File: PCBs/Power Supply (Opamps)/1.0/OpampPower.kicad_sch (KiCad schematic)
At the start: 30 parts, among them J1 Conn_01x02_Male, J2 Conn_01x02_Male, J3 Conn_01x03_Male, J4 Conn_01x03_Male, J5 Conn_01x03_Male, U1 LM317_SOT-223, U2 LM337_SOT223

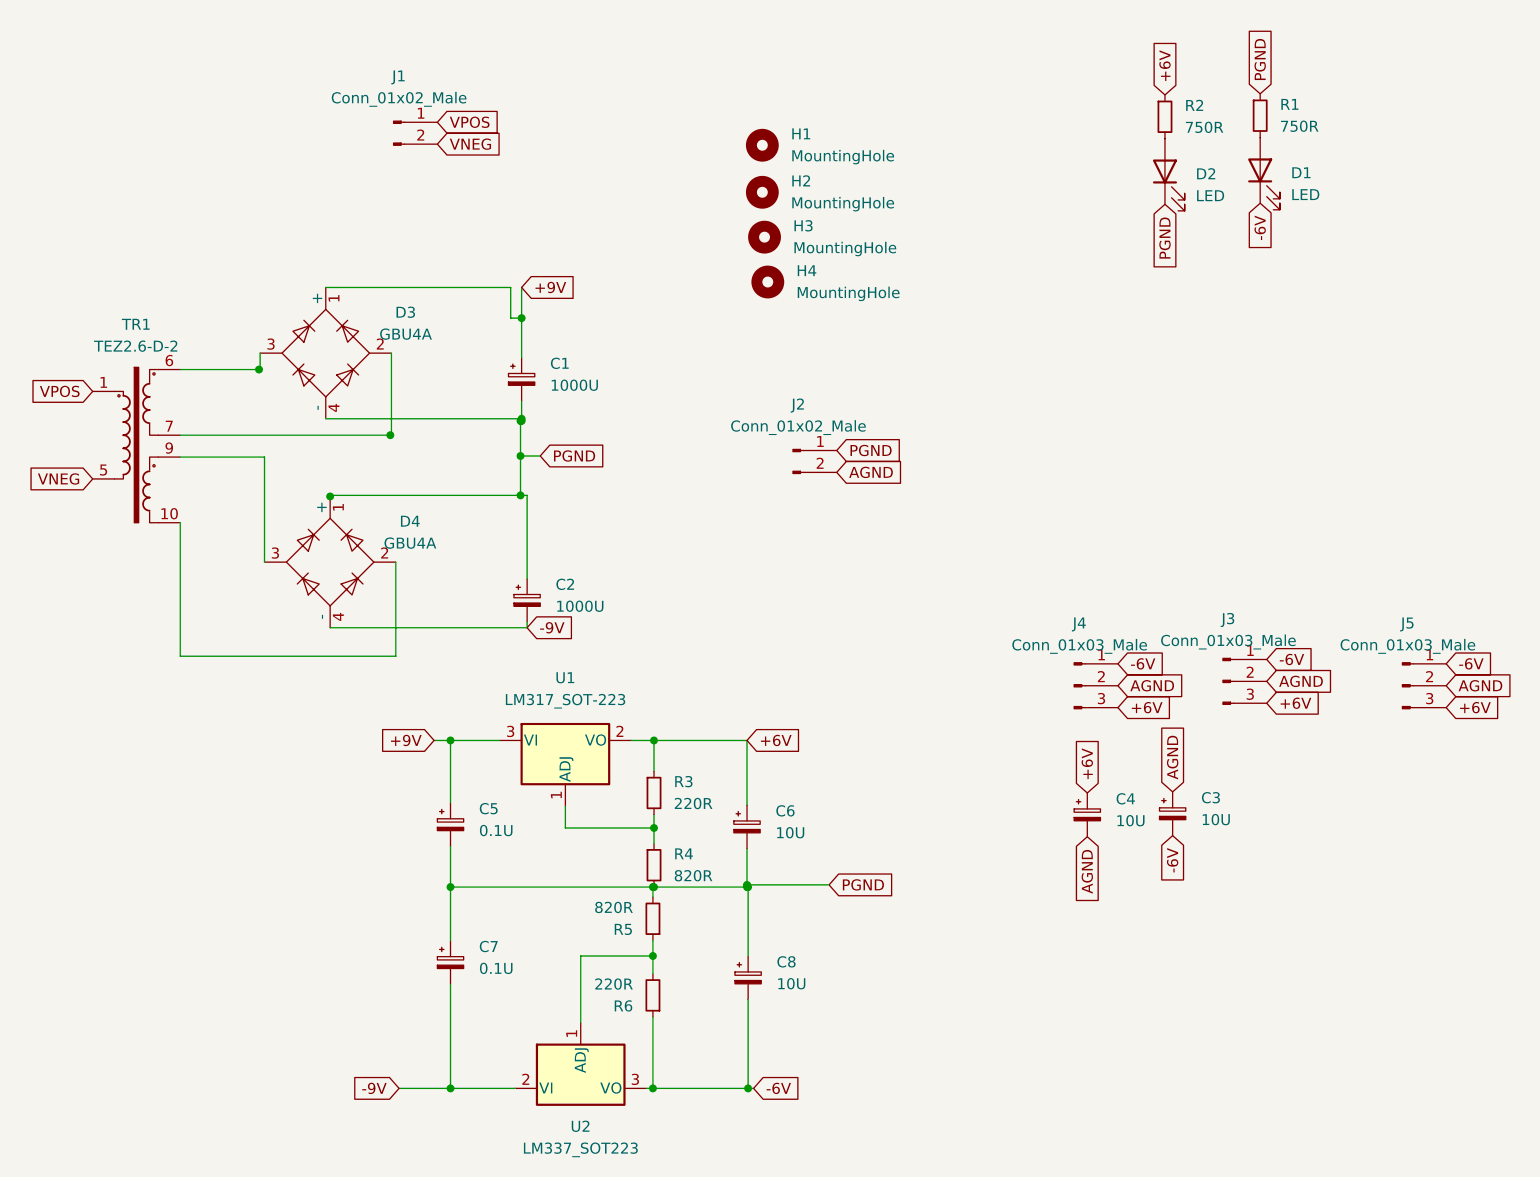
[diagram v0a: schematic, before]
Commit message: Major updates
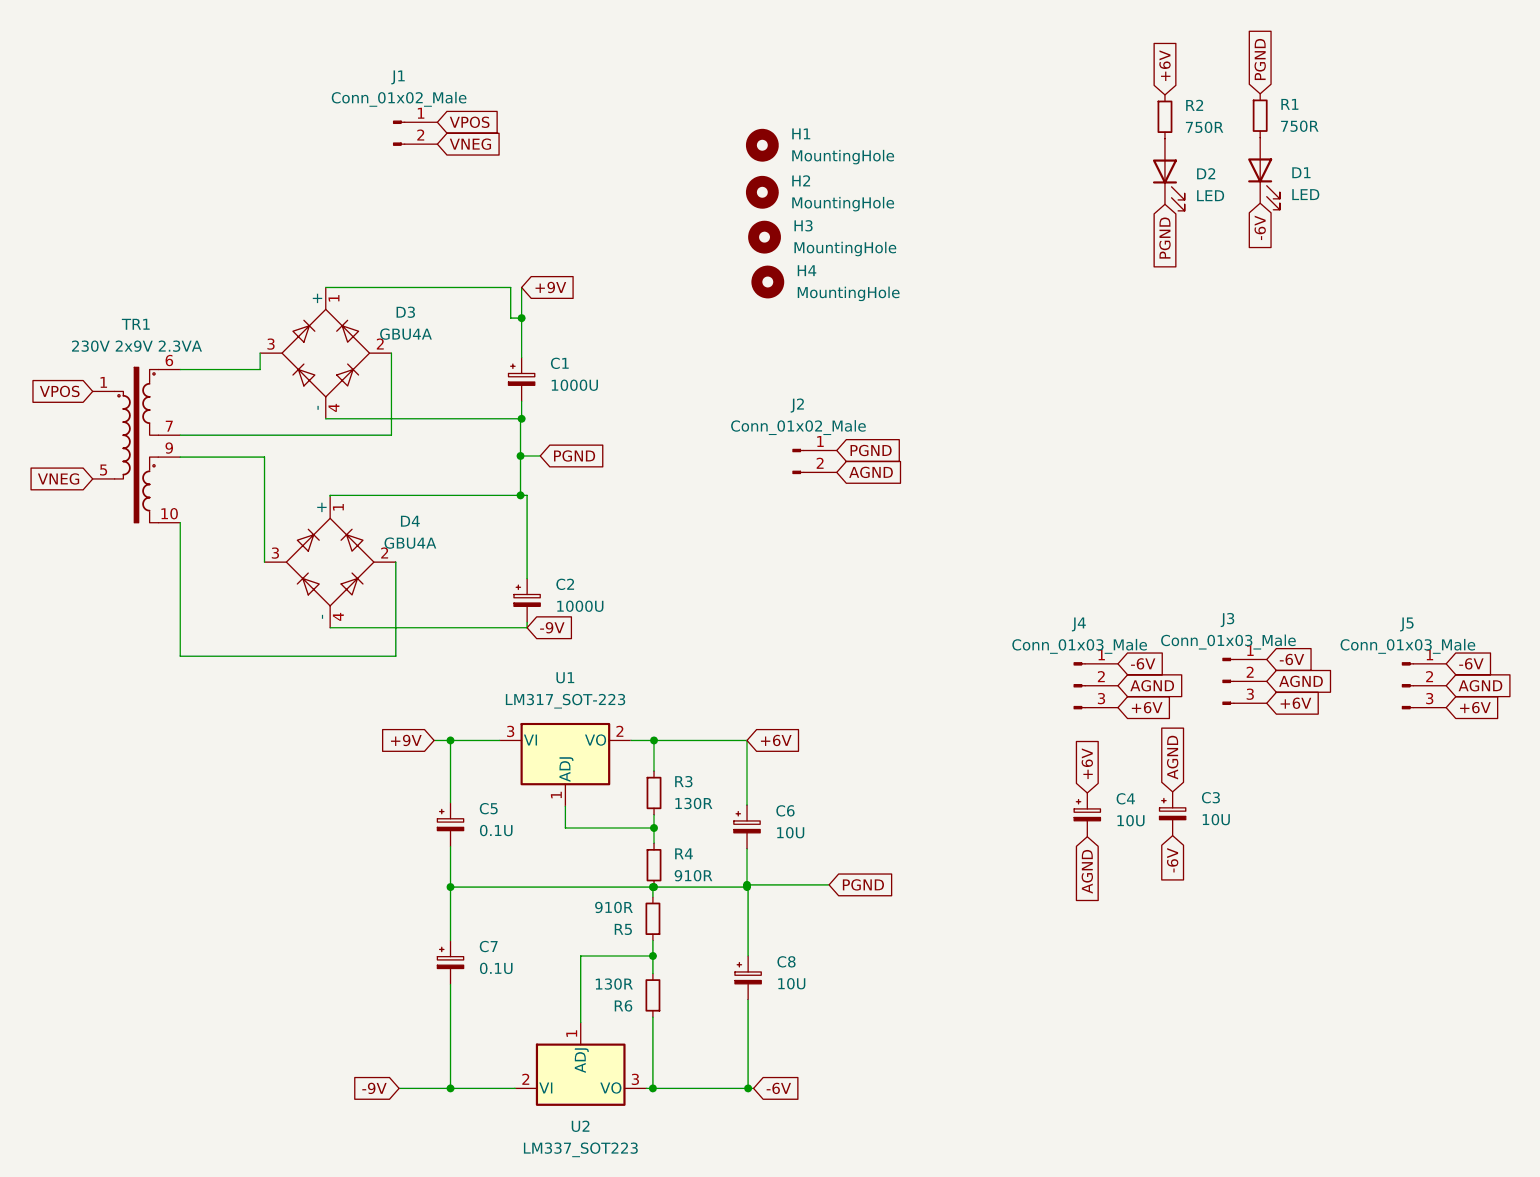
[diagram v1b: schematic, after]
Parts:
- R3, R6: value 220R -> 130R
- R4, R5: value 820R -> 910R
- TR1: value TEZ2.6-D-2 -> 230V 2x9V 2.3VA
